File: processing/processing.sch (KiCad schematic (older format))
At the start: 26 parts, among them J1 HRO-TYPE-C-31-M-12, J2 Conn_01x03, J3 ICSP, SW1 SW_RESET, U1 CH340G, U2 ATmega328P-AU, Y1 12MHz, Y2 16MHz

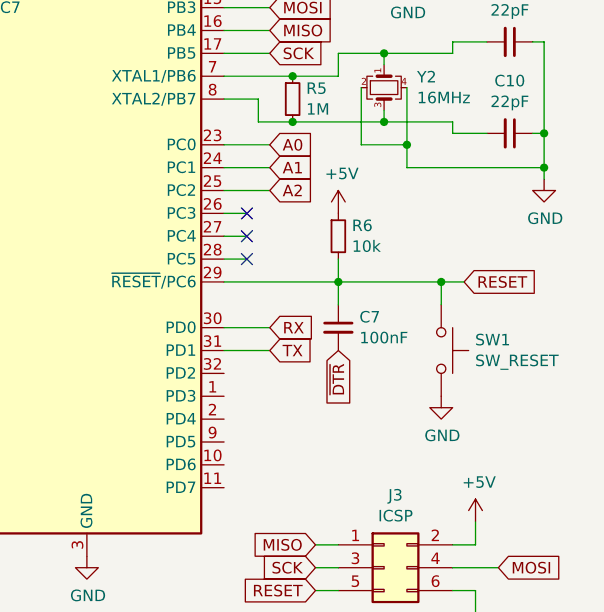
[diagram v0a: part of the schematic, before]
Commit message: base audio board
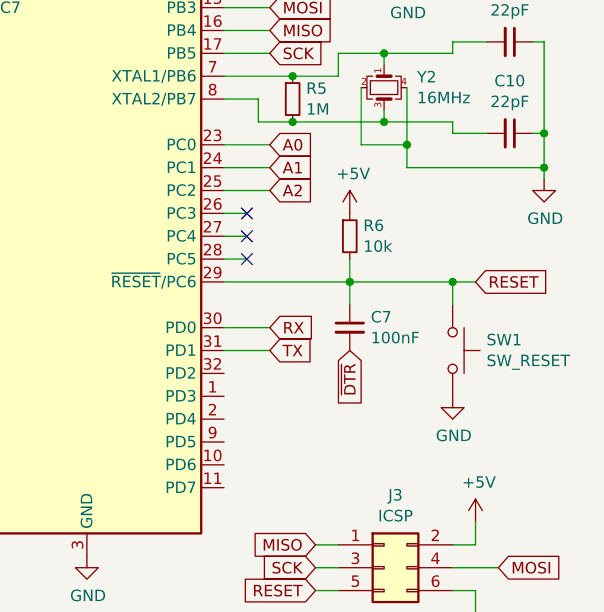
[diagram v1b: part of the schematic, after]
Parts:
- R3, R4: footprint Resistor_SMD:R_1206_3216Metric -> Resistor_SMD:R_0603_1608Metric
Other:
- moved on the sheet: C7, R6, SW1
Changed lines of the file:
@@
 	0    -1   -1   0
 $EndComp
-Wire Wire Line
-	8550 4100 9050 4100
-Wire Wire Line
-	9050 4100 9500 4100
-Connection ~ 9500 4100
-Wire Wire Line
-	9500 4100 9600 4100
-Wire Wire Line
-	9500 4200 9500 4100
-Text GLabel 9600 4100 2    50   Input ~ 0
+Connection ~ 9550 4100
+Wire Wire Line
+	9550 4200 9550 4100
+Text GLabel 9650 4100 2    50   Input ~ 0
 RESET
 $Comp
 L Device:C_Small C7
 U 1 1 60592AFD
-P 9050 4300
-F 0 "C7" H 9142 4346 50  0000 L CNN
-F 1 "100nF" H 9142 4255 50  0000 L CNN
-F 2 "Capacitor_SMD:C_0603_1608Metric" H 9050 4300 50  0001 C CNN
-F 3 "~" H 9050 4300 50  0001 C CNN
-	1    9050 4300
-	1    0    0    -1
-$EndComp
-Text GLabel 9050 4400 3    50   Input ~ 0
+P 9100 4300
+F 0 "C7" H 9192 4346 50  0000 L CNN
+F 1 "100nF" H 9192 4255 50  0000 L CNN
+F 2 "Capacitor_SMD:C_0603_1608Metric" H 9100 4300 50  0001 C CNN
+F 3 "~" H 9100 4300 50  0001 C CNN
+	1    9100 4300
+	1    0    0    -1
+$EndComp
+Text GLabel 9100 4400 3    50   Input ~ 0
 ~DTR
 $Comp
 L Switch:SW_Push SW1
 U 1 1 605744B8
-P 9500 4400
-F 0 "SW1" V 9454 4548 50  0000 L CNN
-F 1 "SW_RESET" V 9545 4548 50  0000 L CNN
-F 2 "Button_Switch_SMD:SW_SPST_SKQG_WithoutStem" H 9500 4600 50  0001 C CNN
-F 3 "~" H 9500 4600 50  0001 C CNN
-	1    9500 4400
+P 9550 4400
+F 0 "SW1" V 9504 4548 50  0000 L CNN
+F 1 "SW_RESET" V 9595 4548 50  0000 L CNN
+F 2 "Button_Switch_SMD:SW_SPST_SKQG_WithoutStem" H 9550 4600 50  0001 C CNN
+F 3 "~" H 9550 4600 50  0001 C CNN
+	1    9550 4400
 	0    1    1    0
 $EndComp
@@
 L power:GND #PWR020
 U 1 1 605B0D83
-P 9500 4600
-F 0 "#PWR020" H 9500 4350 50  0001 C CNN
-F 1 "GND" H 9505 4427 50  0000 C CNN
-F 2 "" H 9500 4600 50  0001 C CNN
-F 3 "" H 9500 4600 50  0001 C CNN
-	1    9500 4600
-	1    0    0    -1
-$EndComp
-Wire Wire Line
-	9050 4200 9050 4100
-Connection ~ 9050 4100
-Wire Wire Line
-	9050 4100 9050 4000
+P 9550 4600
+F 0 "#PWR020" H 9550 4350 50  0001 C CNN
+F 1 "GND" H 9555 4427 50  0000 C CNN
+F 2 "" H 9550 4600 50  0001 C CNN
+F 3 "" H 9550 4600 50  0001 C CNN
+	1    9550 4600
+	1    0    0    -1
+$EndComp
+Wire Wire Line
+	9100 4200 9100 4100
+Connection ~ 9100 4100
+Wire Wire Line
+	9100 4100 9100 4000
 $Comp
 L power:+5V #PWR016
 U 1 1 605738B3
-P 9050 3800
-F 0 "#PWR016" H 9050 3650 50  0001 C CNN
-F 1 "+5V" H 9065 3973 50  0000 C CNN
-F 2 "" H 9050 3800 50  0001 C CNN
-F 3 "" H 9050 3800 50  0001 C CNN
-	1    9050 3800
+P 9100 3800
+F 0 "#PWR016" H 9100 3650 50  0001 C CNN
+F 1 "+5V" H 9115 3973 50  0000 C CNN
+F 2 "" H 9100 3800 50  0001 C CNN
+F 3 "" H 9100 3800 50  0001 C CNN
+	1    9100 3800
 	1    0    0    -1
 $EndComp
@@
 L Device:R_Small R6
 U 1 1 60572FD6
-P 9050 3900
-F 0 "R6" H 9109 3946 50  0000 L CNN
-F 1 "10k" H 9109 3855 50  0000 L CNN
-F 2 "Resistor_SMD:R_1206_3216Metric" H 9050 3900 50  0001 C CNN
-F 3 "~" H 9050 3900 50  0001 C CNN
-	1    9050 3900
+P 9100 3900
+F 0 "R6" H 9159 3946 50  0000 L CNN
+F 1 "10k" H 9159 3855 50  0000 L CNN
+F 2 "Resistor_SMD:R_1206_3216Metric" H 9100 3900 50  0001 C CNN
+F 3 "~" H 9100 3900 50  0001 C CNN
+	1    9100 3900
 	1    0    0    -1
 $EndComp
@@
 F 0 "R3" H 6909 2446 50  0000 L CNN
 F 1 "12k" H 6909 2355 50  0000 L CNN
-F 2 "Resistor_SMD:R_1206_3216Metric" H 6850 2400 50  0001 C CNN
+F 2 "Resistor_SMD:R_0603_1608Metric" H 6850 2400 50  0001 C CNN
 F 3 "~" H 6850 2400 50  0001 C CNN
 	1    6850 2400
@@
 F 0 "R4" H 6909 2846 50  0000 L CNN
 F 1 "8.2k" H 6909 2755 50  0000 L CNN
-F 2 "Resistor_SMD:R_1206_3216Metric" H 6850 2800 50  0001 C CNN
+F 2 "Resistor_SMD:R_0603_1608Metric" H 6850 2800 50  0001 C CNN
 F 3 "~" H 6850 2800 50  0001 C CNN
 	1    6850 2800
@@
 	1    0    0    -1
 $EndComp
+Wire Wire Line
+	9550 4100 9650 4100
+Wire Wire Line
+	9100 4100 9550 4100
+Wire Wire Line
+	8550 4100 9100 4100
 $EndSCHEMATC

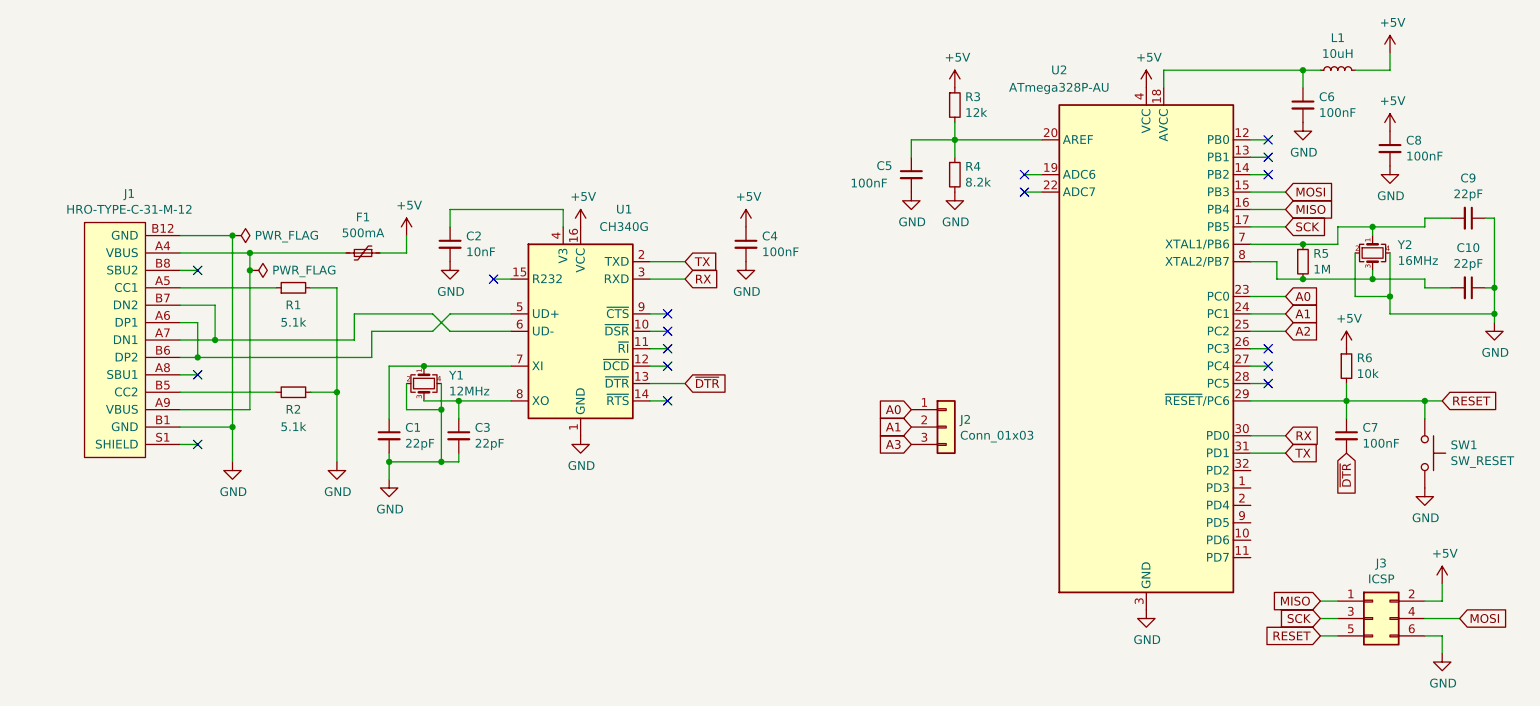
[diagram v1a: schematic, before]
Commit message: finish the processing board
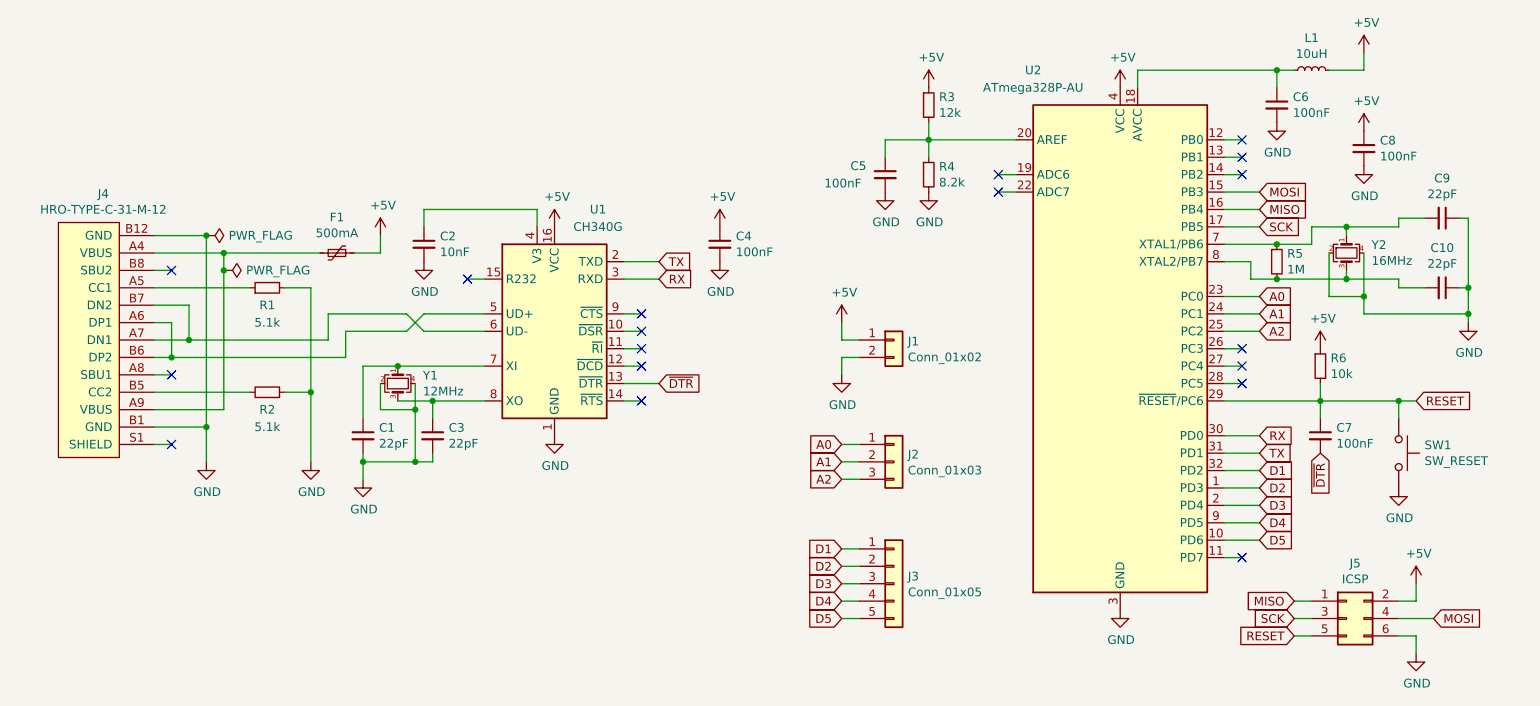
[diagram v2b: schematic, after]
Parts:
- added J1: Conn_01x02, Connector_PinSocket_2.54mm:PinSocket_1x02_P2.54mm_Vertical, symbol Connector_Generic:Conn_01x02
- added J3: Conn_01x05, Connector_PinSocket_2.54mm:PinSocket_1x05_P2.54mm_Vertical, symbol Connector_Generic:Conn_01x05
- J2: footprint Connector_PinHeader_2.54mm:PinHeader_1x03_P2.54mm_Vertical -> Connector_PinSocket_2.54mm:PinSocket_1x03_P2.54mm_Vertical
- renumbered J1 to J4, J3 to J5
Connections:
- net A3 is gone; now on net A2: J2.3 (Pin_3)
- net +5V: now also J1.1 (Pin_1)
- net GND: now also J1.2 (Pin_2)
- net D2: now reaches U2.1 (PD3)
- net D2: now also J3.2 (Pin_2)
- net D5: now reaches U2.10 (PD6)
- net D5: now also J3.5 (Pin_5)
- net D3: now reaches U2.2 (PD4)
- net D3: now also J3.3 (Pin_3)
- net D1: now reaches U2.32 (PD2)
- net D1: now also J3.1 (Pin_1)
- net D4: now reaches U2.9 (PD5)
- net D4: now also J3.4 (Pin_4)
- no-connect marks 17 -> 18
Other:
- moved on the sheet: C1, C10, C2, C3, C4, C5, C6, C7, C8, C9, F1, J2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
